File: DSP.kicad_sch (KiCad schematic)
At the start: 21 parts, among them J10 Conn_01x07_Female, J11 Conn_01x04, Q4 2N3904-SMD, Q5 2N3904-SMD, Q6 AO3400A, SW1 SW_DIP_x01, SW2 Frequency, SW3 Menu, U6 ESP32-A1S

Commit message: gg
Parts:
- C24, C26: footprint Capacitor_SMD:C_1206_3216Metric -> Capacitor_SMD:CP_Elec_4x4.5
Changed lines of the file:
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@@
     (property "Reference" "C26" (id 0) (at 186.69 96.52 90))
     (property "Value" "22uF" (id 1) (at 191.77 96.52 90))
-    (property "Footprint" "Capacitor_SMD:C_1206_3216Metric" (id 2) (at 193.04 99.3648 0)
+    (property "Footprint" "Capacitor_SMD:CP_Elec_4x4.5" (id 2) (at 193.04 99.3648 0)
       (effects (font (size 1.27 1.27)) hide)
     )
@@
     (property "Reference" "C24" (id 0) (at 175.26 106.68 90))
     (property "Value" "22uF" (id 1) (at 180.34 106.68 90))
-    (property "Footprint" "Capacitor_SMD:C_1206_3216Metric" (id 2) (at 182.88 101.9048 0)
-      (effects (font (size 1.27 1.27)) hide)
-    )
+    (property "Footprint" "Capacitor_SMD:CP_Elec_4x4.5" (id 2) (at 182.88 101.9048 0)
+      (effects (font (size 1.27 1.27)) hide)
+    )

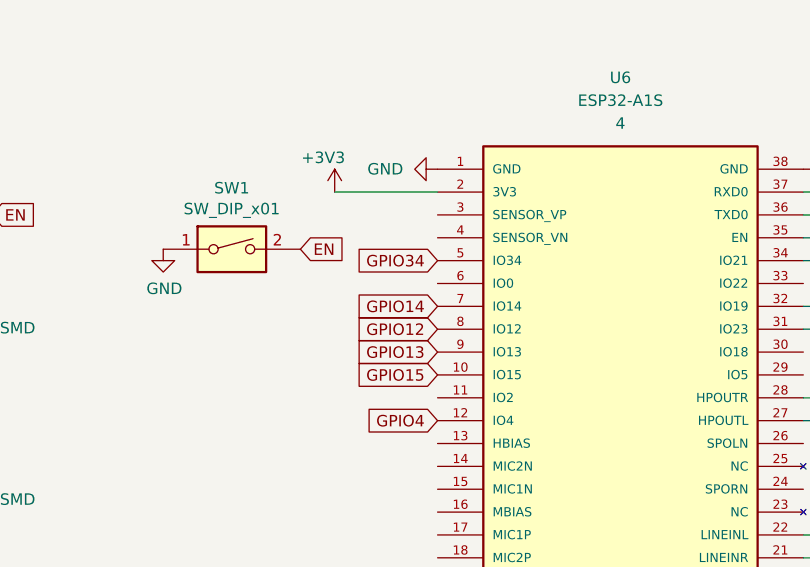
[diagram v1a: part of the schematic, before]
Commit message: gg
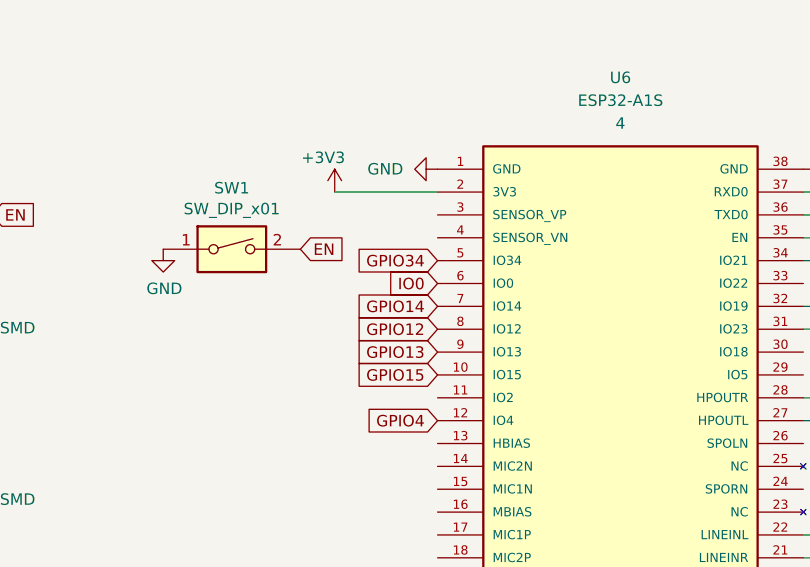
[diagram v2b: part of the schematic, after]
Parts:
- SW1: footprint Button_Switch_THT:SW_PUSH_6mm -> Button_Switch_SMD:SW_SPST_B3U-1000P
- U6: footprint Xenir:ESP32-A1S -> xenir_v6:esp32-a1s-header
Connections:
- net IO0: now also U6.6 (IO0)
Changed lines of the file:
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@@
+    )
+  )
+  (global_label "IO0" (shape input) (at 118.11 87.63 180) (fields_autoplaced)
+    (effects (font (size 1.27 1.27)) (justify right))
+    (property "Intersheet References" "${INTERSHEET_REFS}" (id 0) (at 184.15 318.77 0)
+      (effects (font (size 1.27 1.27)) hide)
     )
   )
@@
     (property "Reference" "SW1" (id 0) (at 95.25 77.0382 0))
     (property "Value" "SW_DIP_x01" (id 1) (at 95.25 79.3496 0))
-    (property "Footprint" "Button_Switch_THT:SW_PUSH_6mm" (id 2) (at 95.25 83.82 0)
+    (property "Footprint" "Button_Switch_SMD:SW_SPST_B3U-1000P" (id 2) (at 95.25 83.82 0)
       (effects (font (size 1.27 1.27)) hide)
     )
@@
     (property "Reference" "U6" (id 0) (at 138.43 64.77 0))
     (property "Value" "ESP32-A1S" (id 1) (at 138.43 67.31 0))
-    (property "Footprint" "Xenir:ESP32-A1S" (id 2) (at 123.19 67.31 0)
+    (property "Footprint" "xenir_v6:esp32-a1s-header" (id 2) (at 123.19 67.31 0)
       (effects (font (size 1.27 1.27)) (justify left bottom) hide)
     )

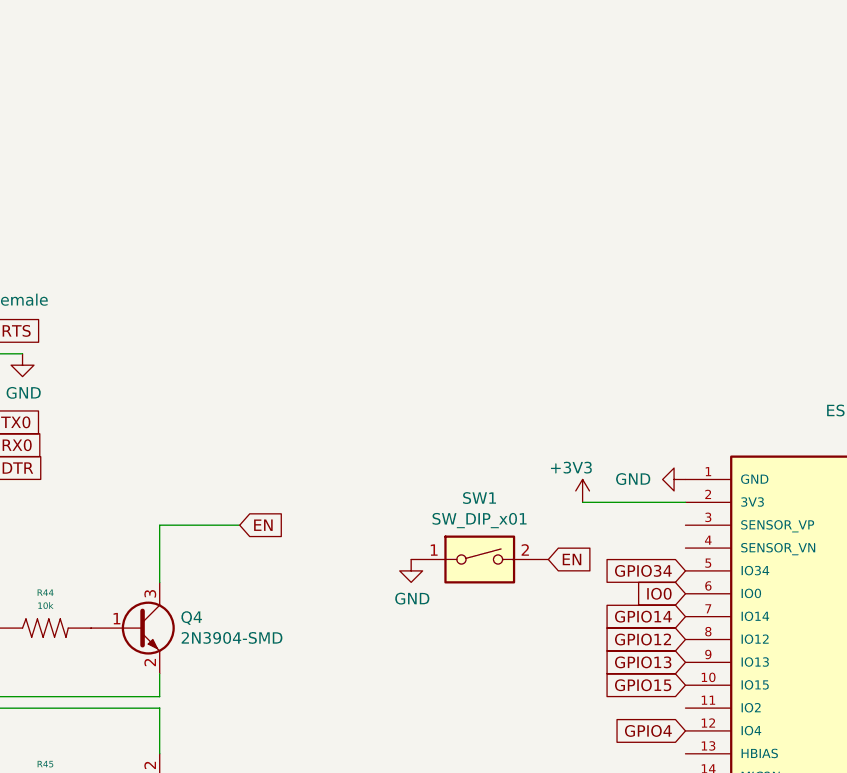
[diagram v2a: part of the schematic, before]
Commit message: gg
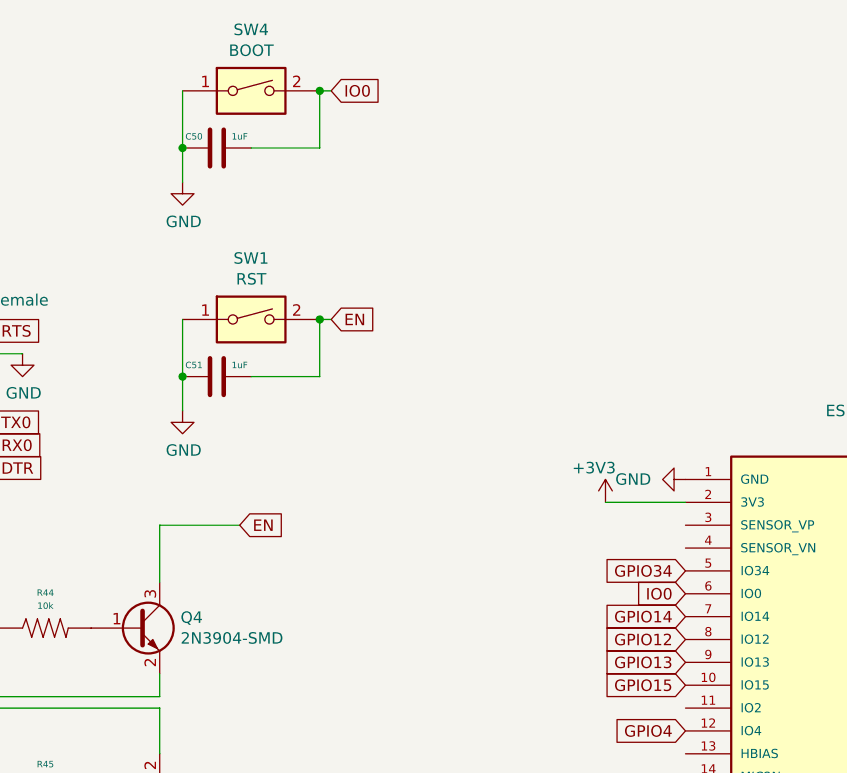
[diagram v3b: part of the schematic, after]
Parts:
- added C50, C51: 1uF, Capacitor_SMD:C_1206_3216Metric, symbol Xenir:Capacitor
- added SW4: BOOT, Button_Switch_SMD:SW_SPST_B3U-1000P, symbol Switch:SW_DIP_x01
- SW1: value SW_DIP_x01 -> RST
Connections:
- net EN: now also C51.2
- net GND: now also C50.1, C51.1, SW4.1
- net IO0: now also C50.2, SW4.2
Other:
- moved on the sheet: SW1
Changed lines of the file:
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@@
 (kicad_sch (version 20211123) (generator eeschema)
   (paper "A4")
+  (junction (at 62.23 63.5) (diameter 0) (color 0 0 0 0)
+  )
+  (junction (at 62.23 38.1) (diameter 0) (color 0 0 0 0)
+  )
   (junction (at 204.47 102.87) (diameter 0) (color 0 0 0 0)
   )
+  (junction (at 77.47 57.15) (diameter 0) (color 0 0 0 0)
+  )
   (junction (at 40.64 91.44) (diameter 0) (color 0 0 0 0)
   )
   (junction (at 214.63 100.33) (diameter 0) (color 0 0 0 0)
   )
+  (junction (at 77.47 31.75) (diameter 0) (color 0 0 0 0)
+  )
   (junction (at 39.37 110.49) (diameter 0) (color 0 0 0 0)
   )
@@
     (stroke (width 0) (type default) (color 0 0 0 0))
   )
+  (wire (pts (xy 77.47 57.15) (xy 77.47 63.5))
+    (stroke (width 0) (type default) (color 0 0 0 0))
+  )
   (wire (pts (xy 59.69 80.01) (xy 68.58 80.01))
     (stroke (width 0) (type default) (color 0 0 0 0))
@@
     (stroke (width 0) (type default) (color 0 0 0 0))
   )
+  (wire (pts (xy 62.23 38.1) (xy 62.23 31.75))
+    (stroke (width 0) (type default) (color 0 0 0 0))
+  )
   (wire (pts (xy 158.75 77.47) (xy 165.1 77.47))
     (stroke (width 0) (type default) (color 0 0 0 0))
@@
     (stroke (width 0) (type default) (color 0 0 0 0))
   )
-  (wire (pts (xy 106.68 77.47) (xy 118.11 77.47))
+  (wire (pts (xy 109.22 77.47) (xy 118.11 77.47))
     (stroke (width 0) (type default) (color 0 0 0 0))
   )
@@
     (stroke (width 0) (type default) (color 0 0 0 0))
   )
+  (wire (pts (xy 77.47 63.5) (xy 69.85 63.5))
+    (stroke (width 0) (type default) (color 0 0 0 0))
+  )
   (wire (pts (xy 158.75 102.87) (xy 175.26 102.87))
     (stroke (width 0) (type default) (color 0 0 0 0))
   )
+  (wire (pts (xy 62.23 67.31) (xy 62.23 63.5))
+    (stroke (width 0) (type default) (color 0 0 0 0))
+  )
   (wire (pts (xy 39.37 110.49) (xy 39.37 99.06))
     (stroke (width 0) (type default) (color 0 0 0 0))
@@
     (stroke (width 0) (type default) (color 0 0 0 0))
   )
+  (wire (pts (xy 62.23 63.5) (xy 62.23 57.15))
+    (stroke (width 0) (type default) (color 0 0 0 0))
+  )
   (wire (pts (xy 40.64 91.44) (xy 41.91 91.44))
     (stroke (width 0) (type default) (color 0 0 0 0))
@@
     (stroke (width 0) (type default) (color 0 0 0 0))
   )
+  (wire (pts (xy 77.47 31.75) (xy 78.74 31.75))
+    (stroke (width 0) (type default) (color 0 0 0 0))
+  )
+  (wire (pts (xy 77.47 57.15) (xy 78.74 57.15))
+    (stroke (width 0) (type default) (color 0 0 0 0))
+  )
   (wire (pts (xy 59.69 100.33) (xy 59.69 105.41))
     (stroke (width 0) (type default) (color 0 0 0 0))
@@
     (stroke (width 0) (type default) (color 0 0 0 0))
   )
+  (wire (pts (xy 62.23 41.91) (xy 62.23 38.1))
+    (stroke (width 0) (type default) (color 0 0 0 0))
+  )
   (wire (pts (xy 186.69 142.24) (xy 194.31 142.24))
     (stroke (width 0) (type default) (color 0 0 0 0))
@@
     (stroke (width 0) (type default) (color 0 0 0 0))
   )
+  (wire (pts (xy 77.47 38.1) (xy 69.85 38.1))
+    (stroke (width 0) (type default) (color 0 0 0 0))
+  )
   (wire (pts (xy 158.75 146.05) (xy 148.59 146.05))
     (stroke (width 0) (type default) (color 0 0 0 0))
   )
   (wire (pts (xy 158.75 82.55) (xy 165.1 82.55))
+    (stroke (width 0) (type default) (color 0 0 0 0))
+  )
+  (wire (pts (xy 77.47 31.75) (xy 77.47 38.1))
     (stroke (width 0) (type default) (color 0 0 0 0))
   )
@@
     )
   )
+  (global_label "IO0" (shape input) (at 78.74 31.75 0) (fields_autoplaced)
+    (effects (font (size 1.27 1.27)) (justify left))
+    (property "Intersheet References" "${INTERSHEET_REFS}" (id 0) (at 12.7 -199.39 0)
+      (effects (font (size 1.27 1.27)) hide)
+    )
+  )
   (global_label "GPIO4" (shape input) (at 133.35 143.51 180) (fields_autoplaced)
     (effects (font (size 1.27 1.27)) (justify right))
@@
     )
   )
-  (global_label "EN" (shape input) (at 102.87 83.82 0) (fields_autoplaced)
-    (effects (font (size 1.27 1.27)) (justify left))
-    (property "Intersheet References" "${INTERSHEET_REFS}" (id 0) (at 2.54 -109.22 0)
+  (global_label "EN" (shape input) (at 78.74 57.15 0) (fields_autoplaced)
+    (effects (font (size 1.27 1.27)) (justify left))
+    (property "Intersheet References" "${INTERSHEET_REFS}" (id 0) (at -21.59 -135.89 0)
       (effects (font (size 1.27 1.27)) hide)
     )
@@
     (pin "2")
   )
-  (symbol (lib_id "Switch:SW_DIP_x01") (at 95.25 83.82 0) (unit 1)
-    (in_bom yes) (on_board yes)
-    (property "Reference" "SW1" (id 0) (at 95.25 77.0382 0))
-    (property "Value" "SW_DIP_x01" (id 1) (at 95.25 79.3496 0))
-    (property "Footprint" "Button_Switch_SMD:SW_SPST_B3U-1000P" (id 2) (at 95.25 83.82 0)
-      (effects (font (size 1.27 1.27)) hide)
-    )
-    (property "Datasheet" "~" (id 3) (at 95.25 83.82 0)
+  (symbol (lib_id "Switch:SW_DIP_x01") (at 69.85 57.15 0) (unit 1)
+    (in_bom yes) (on_board yes)
+    (property "Reference" "SW1" (id 0) (at 69.85 50.3682 0))
+    (property "Value" "RST" (id 1) (at 69.85 52.6796 0))
+    (property "Footprint" "Button_Switch_SMD:SW_SPST_B3U-1000P" (id 2) (at 69.85 57.15 0)
+      (effects (font (size 1.27 1.27)) hide)
+    )
+    (property "Datasheet" "~" (id 3) (at 69.85 57.15 0)
       (effects (font (size 1.27 1.27)) hide)
     )
@@
     (pin "1")
   )
-  (symbol (lib_id "power:+3V3") (at 106.68 77.47 0) (unit 1)
-    (in_bom yes) (on_board yes)
-    (property "Reference" "#PWR0201" (id 0) (at 106.68 81.28 0)
-      (effects (font (size 1.27 1.27)) hide)
-    )
-    (property "Value" "+3V3" (id 1) (at 105.41 73.66 0))
-    (property "Footprint" "" (id 2) (at 106.68 77.47 0)
-      (effects (font (size 1.27 1.27)) hide)
-    )
-    (property "Datasheet" "" (id 3) (at 106.68 77.47 0)
+  (symbol (lib_id "power:+3V3") (at 109.22 77.47 0) (unit 1)
+    (in_bom yes) (on_board yes)
+    (property "Reference" "#PWR0201" (id 0) (at 109.22 81.28 0)
+      (effects (font (size 1.27 1.27)) hide)
+    )
+    (property "Value" "+3V3" (id 1) (at 107.95 73.66 0))
+    (property "Footprint" "" (id 2) (at 109.22 77.47 0)
+      (effects (font (size 1.27 1.27)) hide)
+    )
+    (property "Datasheet" "" (id 3) (at 109.22 77.47 0)
       (effects (font (size 1.27 1.27)) hide)
     )
@@
     (pin "7")
   )
+  (symbol (lib_id "Xenir:Capacitor") (at 66.04 63.5 0) (unit 1)
+    (in_bom yes) (on_board yes)
+    (property "Reference" "C51" (id 0) (at 63.5 62.23 0)
+      (effects (font (size 0.7112 0.7112)))
+    )
+    (property "Value" "1uF" (id 1) (at 68.58 62.23 0)
+      (effects (font (size 0.7112 0.7112)))
+    )
+    (property "Footprint" "Capacitor_SMD:C_1206_3216Metric" (id 2) (at 66.04 67.31 0)
+      (effects (font (size 1.27 1.27)) hide)
+    )
+    (property "Datasheet" "" (id 3) (at 66.04 67.31 0)
+      (effects (font (size 1.27 1.27)) hide)
+    )
+    (pin "1")
+    (pin "2")
+  )
+  (symbol (lib_id "power:GND") (at 62.23 41.91 0) (unit 1)
+    (in_bom yes) (on_board yes)
+    (property "Reference" "#PWR0205" (id 0) (at 62.23 48.26 0)
+      (effects (font (size 1.27 1.27)) hide)
+    )
+    (property "Value" "GND" (id 1) (at 62.357 46.3042 0))
+    (property "Footprint" "" (id 2) (at 62.23 41.91 0)
+      (effects (font (size 1.27 1.27)) hide)
+    )
+    (property "Datasheet" "" (id 3) (at 62.23 41.91 0)
+      (effects (font (size 1.27 1.27)) hide)
+    )
+    (pin "1")
+  )
   (symbol (lib_id "xenir:Resistor") (at 182.88 53.34 0) (unit 1)
     (in_bom yes) (on_board yes) (fields_autoplaced)
@@
     )
     (pin "1")
+  )
+  (symbol (lib_id "Switch:SW_DIP_x01") (at 69.85 31.75 0) (unit 1)
+    (in_bom yes) (on_board yes)
+    (property "Reference" "SW4" (id 0) (at 69.85 24.9682 0))
+    (property "Value" "BOOT" (id 1) (at 69.85 27.2796 0))
+    (property "Footprint" "Button_Switch_SMD:SW_SPST_B3U-1000P" (id 2) (at 69.85 31.75 0)
+      (effects (font (size 1.27 1.27)) hide)
+    )
+    (property "Datasheet" "~" (id 3) (at 69.85 31.75 0)
+      (effects (font (size 1.27 1.27)) hide)
+    )
+    (pin "1")
+    (pin "2")
   )
   (symbol (lib_id "Xenir:Capacitor") (at 204.47 106.68 90) (unit 1)
@@
     (pin "2")
   )
+  (symbol (lib_id "Xenir:Capacitor") (at 66.04 38.1 0) (unit 1)
+    (in_bom yes) (on_board yes)
+    (property "Reference" "C50" (id 0) (at 63.5 36.83 0)
+      (effects (font (size 0.7112 0.7112)))
+    )
+    (property "Value" "1uF" (id 1) (at 68.58 36.83 0)
+      (effects (font (size 0.7112 0.7112)))
+    )
+    (property "Footprint" "Capacitor_SMD:C_1206_3216Metric" (id 2) (at 66.04 41.91 0)
+      (effects (font (size 1.27 1.27)) hide)
+    )
+    (property "Datasheet" "" (id 3) (at 66.04 41.91 0)
+      (effects (font (size 1.27 1.27)) hide)
+    )
+    (pin "1")
+    (pin "2")
+  )
   (symbol (lib_id "power:GND") (at 158.75 120.65 90) (unit 1)
     (in_bom yes) (on_board yes) (fields_autoplaced)
@@
     (pin "1")
   )
-  (symbol (lib_id "power:GND") (at 87.63 83.82 0) (unit 1)
-    (in_bom yes) (on_board yes)
-    (property "Reference" "#PWR0195" (id 0) (at 87.63 90.17 0)
-      (effects (font (size 1.27 1.27)) hide)
-    )
-    (property "Value" "GND" (id 1) (at 87.757 88.2142 0))
-    (property "Footprint" "" (id 2) (at 87.63 83.82 0)
-      (effects (font (size 1.27 1.27)) hide)
-    )
-    (property "Datasheet" "" (id 3) (at 87.63 83.82 0)
-      (effects (font (size 1.27 1.27)) hide)
-    )
+  (symbol (lib_id "power:GND") (at 62.23 67.31 0) (unit 1)
+    (in_bom yes) (on_board yes)
+    (property "Reference" "#PWR0195" (id 0) (at 62.23 73.66 0)
+      (effects (font (size 1.27 1.27)) hide)
+    )
+    (property "Value" "GND" (id 1) (at 62.357 71.7042 0))
+    (property "Footprint" "" (id 2) (at 62.23 67.31 0)
+      (effects (font (size 1.27 1.27)) hide)
+    )
+    (property "Datasheet" "" (id 3) (at 62.23 67.31 0)
+      (effects (font (size 1.27 1.27)) hide)
+    )
